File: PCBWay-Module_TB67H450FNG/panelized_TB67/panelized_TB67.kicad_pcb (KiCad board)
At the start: 2 copper layers, 36.6 x 95.6 mm, 178 parts, among them IC1 Motor_A, IC2 Motor_B, J1 Conn_01x07_Pin, J2 Conn_01x07_Pin

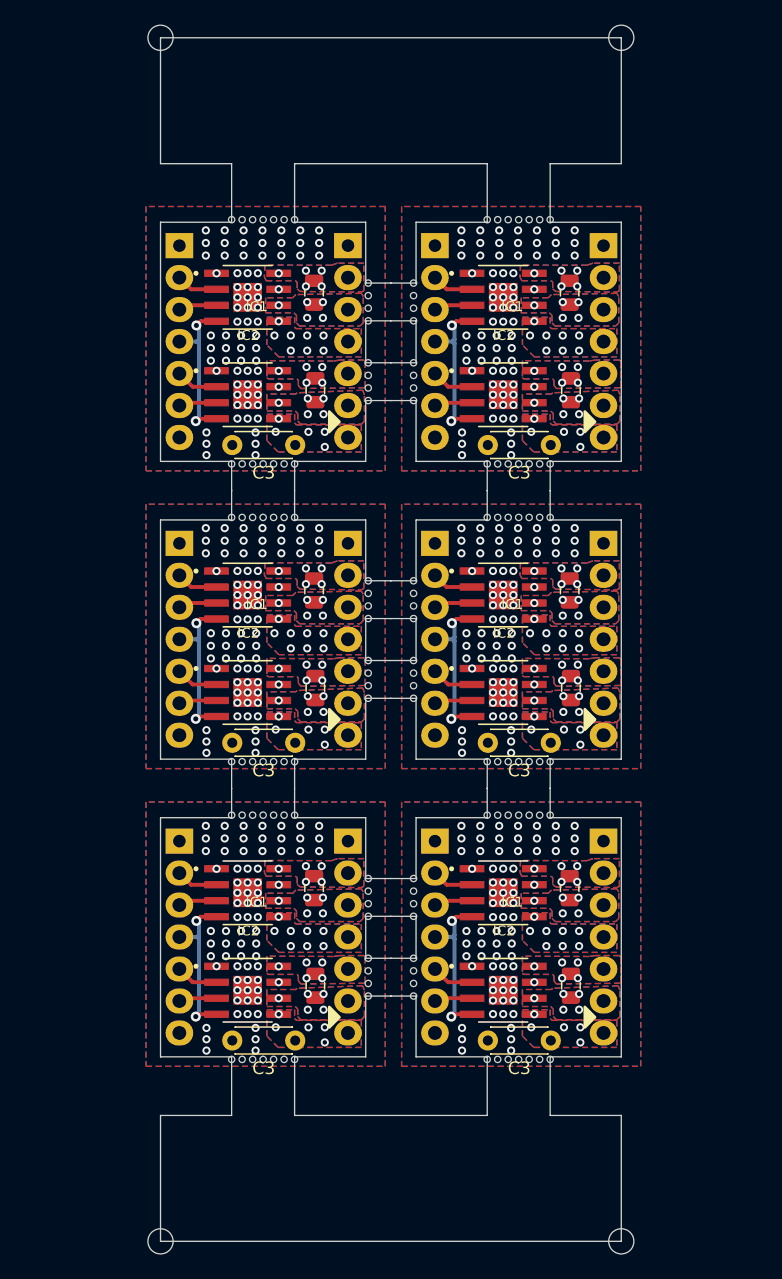
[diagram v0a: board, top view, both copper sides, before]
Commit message: panels
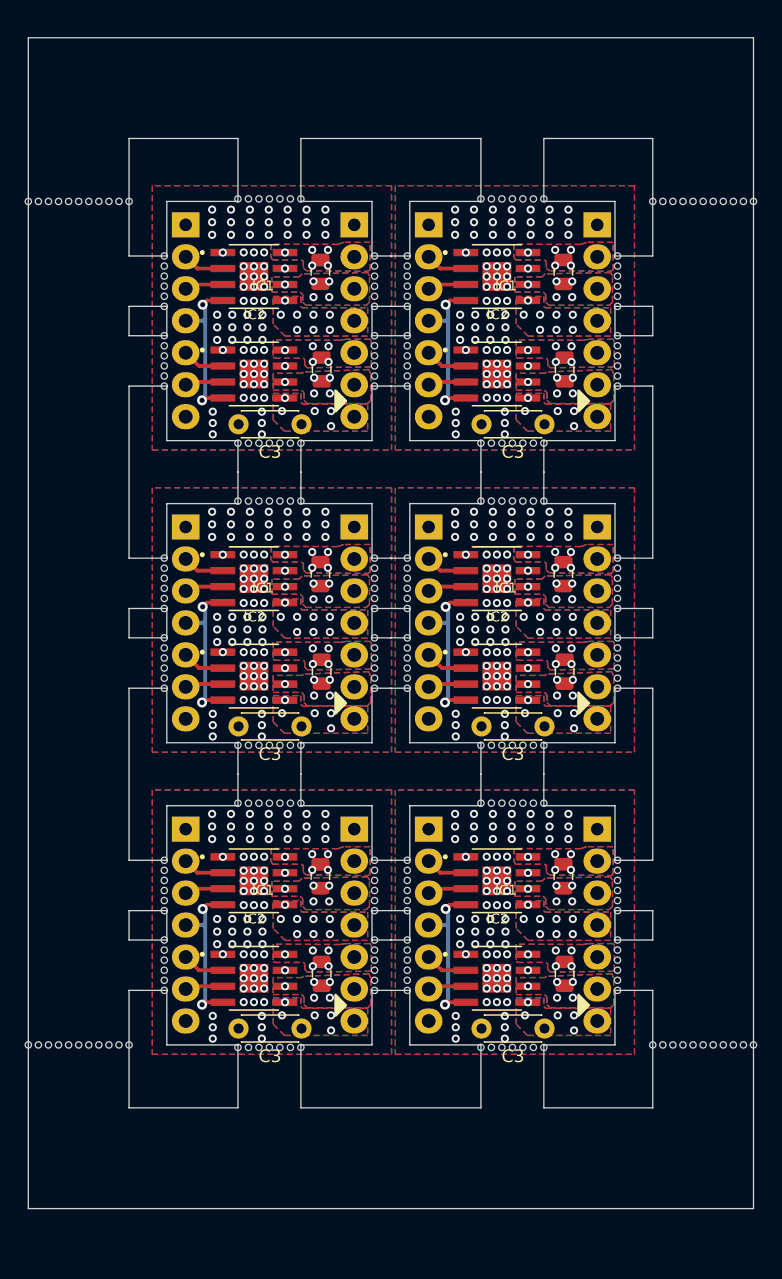
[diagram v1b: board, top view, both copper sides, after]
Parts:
- removed the C1 at (142.5, 95.3)
- removed the C1 at (142.5, 71.7)
- removed the C1 at (162.8, 71.7)
- removed the C1 at (162.8, 48.0)
- removed the C1 at (162.8, 95.3)
- removed the C1 at (142.5, 48.0)
- removed the C2 at (142.4, 63.9)
- removed the C2 at (162.7, 63.9)
- removed the C2 at (142.4, 87.6)
- removed the C2 at (162.7, 87.6)
- removed the C2 at (162.7, 40.3)
- removed the C2 at (142.4, 40.3)
- removed the C3 at (161.2, 52.4)
- removed the C3 at (140.9, 52.4)
- removed the C3 at (140.9, 99.7)
- removed the C3 at (161.2, 76.0)
- removed the C3 at (161.2, 99.7)
- removed the C3 at (140.9, 76.0)
- removed the IC1 at (157.4, 72.0)
- removed the IC1 at (157.4, 48.4)
- removed the IC1 at (157.4, 95.7)
- removed the IC1 at (137.1, 72.0)
- removed the IC1 at (137.1, 48.4)
- removed the IC1 at (137.1, 95.7)
- removed the IC2 at (157.4, 64.3)
- removed the IC2 at (157.4, 87.9)
- removed the IC2 at (137.1, 40.6)
- removed the IC2 at (137.1, 64.3)
- removed the IC2 at (137.1, 87.9)
- removed the IC2 at (157.4, 40.6)
- removed the J1 at (131.7, 36.5)
- removed the J1 at (152.0, 60.2)
- removed the J1 at (131.7, 83.8)
- removed the J1 at (152.0, 83.8)
- removed the J1 at (131.7, 60.2)
- removed the J1 at (152.0, 36.5)
- removed the J2 at (145.1, 36.5)
- removed the J2 at (165.4, 83.8)
- removed the J2 at (145.1, 60.2)
- removed the J2 at (165.4, 36.5)
- removed the J2 at (165.4, 60.2)
- removed the J2 at (145.1, 83.8)
- removed KiKit_MB_15_7, KiKit_MB_16_7, KiKit_MB_19_7, KiKit_MB_20_7, KiKit_MB_3_7, KiKit_MB_4_7, KiKit_MB_7_7, KiKit_MB_8_7, KiKit_TO_1, KiKit_TO_2, KiKit_TO_3, KiKit_TO_4: NPTH, NPTH
- added C1: 100, Capacitor_SMD:C_0805_2012Metric, F.Cu at (143.0, 94.3)
- added C1: 100, Capacitor_SMD:C_0805_2012Metric, F.Cu at (162.3, 94.3)
- added C1: 100, Capacitor_SMD:C_0805_2012Metric, F.Cu at (162.3, 70.3)
- added C1: 100, Capacitor_SMD:C_0805_2012Metric, F.Cu at (143.0, 70.3)
- added C1: 100, Capacitor_SMD:C_0805_2012Metric, F.Cu at (162.3, 46.4)
- added C1: 100, Capacitor_SMD:C_0805_2012Metric, F.Cu at (143.0, 46.4)
- added C2: 100, Capacitor_SMD:C_0805_2012Metric, F.Cu at (162.2, 62.6)
- added C2: 100, Capacitor_SMD:C_0805_2012Metric, F.Cu at (142.9, 86.6)
- added C2: 100, Capacitor_SMD:C_0805_2012Metric, F.Cu at (142.9, 38.6)
- added C2: 100, Capacitor_SMD:C_0805_2012Metric, F.Cu at (162.2, 38.6)
- added C2: 100, Capacitor_SMD:C_0805_2012Metric, F.Cu at (142.9, 62.6)
- added C2: 100, Capacitor_SMD:C_0805_2012Metric, F.Cu at (162.2, 86.6)
- added C3: 100, Capacitor_THT:C_Disc_D4.3mm_W1.9mm_P5.00mm, F.Cu at (160.7, 74.7)
- added C3: 100, Capacitor_THT:C_Disc_D4.3mm_W1.9mm_P5.00mm, F.Cu at (141.4, 98.7)
- added C3: 100, Capacitor_THT:C_Disc_D4.3mm_W1.9mm_P5.00mm, F.Cu at (141.4, 74.7)
- added C3: 100, Capacitor_THT:C_Disc_D4.3mm_W1.9mm_P5.00mm, F.Cu at (141.4, 50.7)
- added C3: 100, Capacitor_THT:C_Disc_D4.3mm_W1.9mm_P5.00mm, F.Cu at (160.7, 50.7)
- added C3: 100, Capacitor_THT:C_Disc_D4.3mm_W1.9mm_P5.00mm, F.Cu at (160.7, 98.7)
- added IC1: Motor_A, TB67H450FNG_EL:TB67H450FNG_EL, F.Cu at (137.6, 94.7)
- added IC1: Motor_A, TB67H450FNG_EL:TB67H450FNG_EL, F.Cu at (156.9, 94.7)
- added IC1: Motor_A, TB67H450FNG_EL:TB67H450FNG_EL, F.Cu at (137.6, 46.7)
- added IC1: Motor_A, TB67H450FNG_EL:TB67H450FNG_EL, F.Cu at (156.9, 70.7)
- added IC1: Motor_A, TB67H450FNG_EL:TB67H450FNG_EL, F.Cu at (156.9, 46.7)
- added IC1: Motor_A, TB67H450FNG_EL:TB67H450FNG_EL, F.Cu at (137.6, 70.7)
- added IC2: Motor_B, TB67H450FNG_EL:TB67H450FNG_EL, F.Cu at (156.9, 39.0)
- added IC2: Motor_B, TB67H450FNG_EL:TB67H450FNG_EL, F.Cu at (156.9, 87.0)
- added IC2: Motor_B, TB67H450FNG_EL:TB67H450FNG_EL, F.Cu at (137.6, 39.0)
- added IC2: Motor_B, TB67H450FNG_EL:TB67H450FNG_EL, F.Cu at (137.6, 87.0)
- added IC2: Motor_B, TB67H450FNG_EL:TB67H450FNG_EL, F.Cu at (156.9, 63.0)
- added IC2: Motor_B, TB67H450FNG_EL:TB67H450FNG_EL, F.Cu at (137.6, 63.0)
- added J1: Conn_01x07_Pin, Connector_PinHeader_2.54mm:PinHeader_1x07_P2.54mm_Vertical, B.Cu at (151.5, 58.9)
- added J1: Conn_01x07_Pin, Connector_PinHeader_2.54mm:PinHeader_1x07_P2.54mm_Vertical, B.Cu at (132.2, 82.9)
- added J1: Conn_01x07_Pin, Connector_PinHeader_2.54mm:PinHeader_1x07_P2.54mm_Vertical, B.Cu at (151.5, 82.9)
- added J1: Conn_01x07_Pin, Connector_PinHeader_2.54mm:PinHeader_1x07_P2.54mm_Vertical, B.Cu at (132.2, 34.9)
- added J1: Conn_01x07_Pin, Connector_PinHeader_2.54mm:PinHeader_1x07_P2.54mm_Vertical, B.Cu at (151.5, 34.9)
- added J1: Conn_01x07_Pin, Connector_PinHeader_2.54mm:PinHeader_1x07_P2.54mm_Vertical, B.Cu at (132.2, 58.9)
- added J2: Conn_01x07_Pin, Connector_PinHeader_2.54mm:PinHeader_1x07_P2.54mm_Vertical, B.Cu at (164.9, 82.9)
- added J2: Conn_01x07_Pin, Connector_PinHeader_2.54mm:PinHeader_1x07_P2.54mm_Vertical, B.Cu at (145.6, 82.9)
- added J2: Conn_01x07_Pin, Connector_PinHeader_2.54mm:PinHeader_1x07_P2.54mm_Vertical, B.Cu at (145.6, 58.9)
- added J2: Conn_01x07_Pin, Connector_PinHeader_2.54mm:PinHeader_1x07_P2.54mm_Vertical, B.Cu at (164.9, 34.9)
- added J2: Conn_01x07_Pin, Connector_PinHeader_2.54mm:PinHeader_1x07_P2.54mm_Vertical, B.Cu at (145.6, 34.9)
- added J2: Conn_01x07_Pin, Connector_PinHeader_2.54mm:PinHeader_1x07_P2.54mm_Vertical, B.Cu at (164.9, 58.9)
- added KiKit_MB_10_5: NPTH, NPTH, F.Cu at (166.5, 46.9)
- added KiKit_MB_10_6: NPTH, NPTH, F.Cu at (166.5, 47.7)
- added KiKit_MB_13_5: NPTH, NPTH, F.Cu at (130.5, 62.1)
- added KiKit_MB_13_6: NPTH, NPTH, F.Cu at (130.5, 61.3)
- added KiKit_MB_14_5: NPTH, NPTH, F.Cu at (130.5, 68.5)
- added KiKit_MB_14_6: NPTH, NPTH, F.Cu at (130.5, 67.7)
- added KiKit_MB_17_5: NPTH, NPTH, F.Cu at (139.7, 56.8)
- added KiKit_MB_17_6: NPTH, NPTH, F.Cu at (140.5, 56.8)
- added KiKit_MB_17_7: NPTH, NPTH, F.Cu at (141.3, 56.8)
- added KiKit_MB_18_5: NPTH, NPTH, F.Cu at (138.0, 76.2)
- added KiKit_MB_18_6: NPTH, NPTH, F.Cu at (137.2, 76.2)
- added KiKit_MB_18_7: NPTH, NPTH, F.Cu at (136.3, 76.2)
- added KiKit_MB_1_5: NPTH, NPTH, F.Cu at (130.5, 38.1)
- added KiKit_MB_1_6: NPTH, NPTH, F.Cu at (130.5, 37.3)
- added KiKit_MB_21_5: NPTH, NPTH, F.Cu at (166.5, 64.5)
- added KiKit_MB_21_6: NPTH, NPTH, F.Cu at (166.5, 65.3)
- added KiKit_MB_22_5: NPTH, NPTH, F.Cu at (166.5, 70.9)
- added KiKit_MB_22_6: NPTH, NPTH, F.Cu at (166.5, 71.7)
- added KiKit_MB_25_1: NPTH, NPTH, F.Cu at (130.5, 89.3)
- added KiKit_MB_25_2: NPTH, NPTH, F.Cu at (130.5, 88.5)
- added KiKit_MB_25_3: NPTH, NPTH, F.Cu at (130.5, 87.7)
- added KiKit_MB_25_4: NPTH, NPTH, F.Cu at (130.5, 86.9)
- added KiKit_MB_25_5: NPTH, NPTH, F.Cu at (130.5, 86.1)
- added KiKit_MB_25_6: NPTH, NPTH, F.Cu at (130.5, 85.3)
- added KiKit_MB_26_1: NPTH, NPTH, F.Cu at (130.5, 95.7)
- added KiKit_MB_26_2: NPTH, NPTH, F.Cu at (130.5, 94.9)
- added KiKit_MB_26_3: NPTH, NPTH, F.Cu at (130.5, 94.1)
- added KiKit_MB_26_4: NPTH, NPTH, F.Cu at (130.5, 93.3)
- added KiKit_MB_26_5: NPTH, NPTH, F.Cu at (130.5, 92.5)
- added KiKit_MB_26_6: NPTH, NPTH, F.Cu at (130.5, 91.7)
- added KiKit_MB_27_1: NPTH, NPTH, F.Cu at (147.2, 85.3)
- added KiKit_MB_27_2: NPTH, NPTH, F.Cu at (147.2, 86.1)
- added KiKit_MB_27_3: NPTH, NPTH, F.Cu at (147.2, 86.9)
- added KiKit_MB_27_4: NPTH, NPTH, F.Cu at (147.2, 87.7)
- added KiKit_MB_27_5: NPTH, NPTH, F.Cu at (147.2, 88.5)
- added KiKit_MB_27_6: NPTH, NPTH, F.Cu at (147.2, 89.3)
- added KiKit_MB_28_1: NPTH, NPTH, F.Cu at (147.2, 91.7)
- added KiKit_MB_28_2: NPTH, NPTH, F.Cu at (147.2, 92.5)
- added KiKit_MB_28_3: NPTH, NPTH, F.Cu at (147.2, 93.3)
- added KiKit_MB_28_4: NPTH, NPTH, F.Cu at (147.2, 94.1)
- added KiKit_MB_28_5: NPTH, NPTH, F.Cu at (147.2, 94.9)
- added KiKit_MB_28_6: NPTH, NPTH, F.Cu at (147.2, 95.7)
- added KiKit_MB_29_1: NPTH, NPTH, F.Cu at (136.3, 80.8)
- added KiKit_MB_29_2: NPTH, NPTH, F.Cu at (137.2, 80.8)
- added KiKit_MB_29_3: NPTH, NPTH, F.Cu at (138.0, 80.8)
- added KiKit_MB_29_4: NPTH, NPTH, F.Cu at (138.8, 80.8)
- added KiKit_MB_29_5: NPTH, NPTH, F.Cu at (139.7, 80.8)
- added KiKit_MB_29_6: NPTH, NPTH, F.Cu at (140.5, 80.8)
- added KiKit_MB_29_7: NPTH, NPTH, F.Cu at (141.3, 80.8)
- added KiKit_MB_2_5: NPTH, NPTH, F.Cu at (130.5, 44.5)
- added KiKit_MB_2_6: NPTH, NPTH, F.Cu at (130.5, 43.7)
- added KiKit_MB_30_1: NPTH, NPTH, F.Cu at (141.3, 100.2)
- added KiKit_MB_30_2: NPTH, NPTH, F.Cu at (140.5, 100.2)
- added KiKit_MB_30_3: NPTH, NPTH, F.Cu at (139.7, 100.2)
- added KiKit_MB_30_4: NPTH, NPTH, F.Cu at (138.8, 100.2)
- added KiKit_MB_30_5: NPTH, NPTH, F.Cu at (138.0, 100.2)
- added KiKit_MB_30_6: NPTH, NPTH, F.Cu at (137.2, 100.2)
- added KiKit_MB_30_7: NPTH, NPTH, F.Cu at (136.3, 100.2)
- added KiKit_MB_31_1: NPTH, NPTH, F.Cu at (149.8, 89.3)
- added KiKit_MB_31_2: NPTH, NPTH, F.Cu at (149.8, 88.5)
- added KiKit_MB_31_3: NPTH, NPTH, F.Cu at (149.8, 87.7)
- added KiKit_MB_31_4: NPTH, NPTH, F.Cu at (149.8, 86.9)
- added KiKit_MB_31_5: NPTH, NPTH, F.Cu at (149.8, 86.1)
- added KiKit_MB_31_6: NPTH, NPTH, F.Cu at (149.8, 85.3)
- added KiKit_MB_32_1: NPTH, NPTH, F.Cu at (149.8, 95.7)
- added KiKit_MB_32_2: NPTH, NPTH, F.Cu at (149.8, 94.9)
- added KiKit_MB_32_3: NPTH, NPTH, F.Cu at (149.8, 94.1)
- added KiKit_MB_32_4: NPTH, NPTH, F.Cu at (149.8, 93.3)
- added KiKit_MB_32_5: NPTH, NPTH, F.Cu at (149.8, 92.5)
- added KiKit_MB_32_6: NPTH, NPTH, F.Cu at (149.8, 91.7)
- added KiKit_MB_33_1: NPTH, NPTH, F.Cu at (166.5, 85.3)
- added KiKit_MB_33_2: NPTH, NPTH, F.Cu at (166.5, 86.1)
- added KiKit_MB_33_3: NPTH, NPTH, F.Cu at (166.5, 86.9)
- added KiKit_MB_33_4: NPTH, NPTH, F.Cu at (166.5, 87.7)
- added KiKit_MB_33_5: NPTH, NPTH, F.Cu at (166.5, 88.5)
- added KiKit_MB_33_6: NPTH, NPTH, F.Cu at (166.5, 89.3)
- added KiKit_MB_34_1: NPTH, NPTH, F.Cu at (166.5, 91.7)
- added KiKit_MB_34_2: NPTH, NPTH, F.Cu at (166.5, 92.5)
- added KiKit_MB_34_3: NPTH, NPTH, F.Cu at (166.5, 93.3)
- added KiKit_MB_34_4: NPTH, NPTH, F.Cu at (166.5, 94.1)
- added KiKit_MB_34_5: NPTH, NPTH, F.Cu at (166.5, 94.9)
- added KiKit_MB_34_6: NPTH, NPTH, F.Cu at (166.5, 95.7)
- added KiKit_MB_35_1: NPTH, NPTH, F.Cu at (155.7, 80.8)
- added KiKit_MB_35_2: NPTH, NPTH, F.Cu at (156.5, 80.8)
- added KiKit_MB_35_3: NPTH, NPTH, F.Cu at (157.3, 80.8)
- added KiKit_MB_35_4: NPTH, NPTH, F.Cu at (158.2, 80.8)
- added KiKit_MB_35_5: NPTH, NPTH, F.Cu at (159.0, 80.8)
- added KiKit_MB_35_6: NPTH, NPTH, F.Cu at (159.8, 80.8)
- added KiKit_MB_35_7: NPTH, NPTH, F.Cu at (160.7, 80.8)
- added KiKit_MB_36_1: NPTH, NPTH, F.Cu at (160.7, 100.2)
- added KiKit_MB_36_2: NPTH, NPTH, F.Cu at (159.8, 100.2)
- added KiKit_MB_36_3: NPTH, NPTH, F.Cu at (159.0, 100.2)
- added KiKit_MB_36_4: NPTH, NPTH, F.Cu at (158.2, 100.2)
- added KiKit_MB_36_5: NPTH, NPTH, F.Cu at (157.3, 100.2)
- added KiKit_MB_36_6: NPTH, NPTH, F.Cu at (156.5, 100.2)
- added KiKit_MB_36_7: NPTH, NPTH, F.Cu at (155.7, 100.2)
- added KiKit_MB_37_1: NPTH, NPTH, F.Cu at (119.7, 33.0)
- added KiKit_MB_37_10: NPTH, NPTH, F.Cu at (126.9, 33.0)
- added KiKit_MB_37_11: NPTH, NPTH, F.Cu at (127.7, 33.0)
- added KiKit_MB_37_2: NPTH, NPTH, F.Cu at (120.5, 33.0)
- added KiKit_MB_37_3: NPTH, NPTH, F.Cu at (121.3, 33.0)
- added KiKit_MB_37_4: NPTH, NPTH, F.Cu at (122.1, 33.0)
- added KiKit_MB_37_5: NPTH, NPTH, F.Cu at (122.9, 33.0)
- added KiKit_MB_37_6: NPTH, NPTH, F.Cu at (123.7, 33.0)
- added KiKit_MB_37_7: NPTH, NPTH, F.Cu at (124.5, 33.0)
- added KiKit_MB_37_8: NPTH, NPTH, F.Cu at (125.3, 33.0)
- added KiKit_MB_37_9: NPTH, NPTH, F.Cu at (126.1, 33.0)
- added KiKit_MB_38_1: NPTH, NPTH, F.Cu at (119.7, 100.0)
- added KiKit_MB_38_10: NPTH, NPTH, F.Cu at (126.9, 100.0)
- added KiKit_MB_38_11: NPTH, NPTH, F.Cu at (127.7, 100.0)
- added KiKit_MB_38_2: NPTH, NPTH, F.Cu at (120.5, 100.0)
- added KiKit_MB_38_3: NPTH, NPTH, F.Cu at (121.3, 100.0)
- added KiKit_MB_38_4: NPTH, NPTH, F.Cu at (122.1, 100.0)
- added KiKit_MB_38_5: NPTH, NPTH, F.Cu at (122.9, 100.0)
- added KiKit_MB_38_6: NPTH, NPTH, F.Cu at (123.7, 100.0)
- added KiKit_MB_38_7: NPTH, NPTH, F.Cu at (124.5, 100.0)
- added KiKit_MB_38_8: NPTH, NPTH, F.Cu at (125.3, 100.0)
- added KiKit_MB_38_9: NPTH, NPTH, F.Cu at (126.1, 100.0)
- added KiKit_MB_39_1: NPTH, NPTH, F.Cu at (169.3, 33.0)
- added KiKit_MB_39_10: NPTH, NPTH, F.Cu at (176.5, 33.0)
- added KiKit_MB_39_11: NPTH, NPTH, F.Cu at (177.3, 33.0)
- added KiKit_MB_39_2: NPTH, NPTH, F.Cu at (170.1, 33.0)
- added KiKit_MB_39_3: NPTH, NPTH, F.Cu at (170.9, 33.0)
- added KiKit_MB_39_4: NPTH, NPTH, F.Cu at (171.7, 33.0)
- added KiKit_MB_39_5: NPTH, NPTH, F.Cu at (172.5, 33.0)
- added KiKit_MB_39_6: NPTH, NPTH, F.Cu at (173.3, 33.0)
- added KiKit_MB_39_7: NPTH, NPTH, F.Cu at (174.1, 33.0)
- added KiKit_MB_39_8: NPTH, NPTH, F.Cu at (174.9, 33.0)
- added KiKit_MB_39_9: NPTH, NPTH, F.Cu at (175.7, 33.0)
- added KiKit_MB_40_1: NPTH, NPTH, F.Cu at (169.3, 100.0)
- added KiKit_MB_40_10: NPTH, NPTH, F.Cu at (176.5, 100.0)
- added KiKit_MB_40_11: NPTH, NPTH, F.Cu at (177.3, 100.0)
- added KiKit_MB_40_2: NPTH, NPTH, F.Cu at (170.1, 100.0)
- added KiKit_MB_40_3: NPTH, NPTH, F.Cu at (170.9, 100.0)
- added KiKit_MB_40_4: NPTH, NPTH, F.Cu at (171.7, 100.0)
- added KiKit_MB_40_5: NPTH, NPTH, F.Cu at (172.5, 100.0)
- added KiKit_MB_40_6: NPTH, NPTH, F.Cu at (173.3, 100.0)
- added KiKit_MB_40_7: NPTH, NPTH, F.Cu at (174.1, 100.0)
- added KiKit_MB_40_8: NPTH, NPTH, F.Cu at (174.9, 100.0)
- added KiKit_MB_40_9: NPTH, NPTH, F.Cu at (175.7, 100.0)
- added KiKit_MB_5_5: NPTH, NPTH, F.Cu at (139.7, 32.8)
- added KiKit_MB_5_6: NPTH, NPTH, F.Cu at (140.5, 32.8)
- added KiKit_MB_5_7: NPTH, NPTH, F.Cu at (141.3, 32.8)
- added KiKit_MB_6_5: NPTH, NPTH, F.Cu at (138.0, 52.2)
- added KiKit_MB_6_6: NPTH, NPTH, F.Cu at (137.2, 52.2)
- added KiKit_MB_6_7: NPTH, NPTH, F.Cu at (136.3, 52.2)
- added KiKit_MB_9_5: NPTH, NPTH, F.Cu at (166.5, 40.5)
- added KiKit_MB_9_6: NPTH, NPTH, F.Cu at (166.5, 41.3)
- moved KiKit_MB_20_6 36.0 mm to (149.8, 67.7)
- moved KiKit_MB_20_5 34.9 mm to (149.8, 68.5)
- moved KiKit_MB_17_4 33.9 mm to (138.8, 56.8)
- moved KiKit_MB_20_4 33.9 mm to (149.8, 69.3)
- moved KiKit_MB_17_3 33.1 mm to (138.0, 56.8)
- moved KiKit_MB_10_4 33.0 mm to (166.5, 46.1)
- moved KiKit_MB_9_4 33.0 mm to (166.5, 39.7)
- moved KiKit_MB_20_3 32.8 mm to (149.8, 70.1)
- moved KiKit_MB_10_3 32.8 mm to (166.5, 45.3)
- moved KiKit_MB_9_3 32.8 mm to (166.5, 38.9)
- moved KiKit_MB_21_1 32.7 mm to (166.5, 61.3)
- moved KiKit_MB_22_1 32.7 mm to (166.5, 67.7)
- moved KiKit_MB_10_2 32.7 mm to (166.5, 44.5)
- moved KiKit_MB_9_2 32.7 mm to (166.5, 38.1)
- moved KiKit_MB_10_1 32.5 mm to (166.5, 43.7)
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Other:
- board size 36.6 x 95.6 mm -> 57.6 x 93 mm
